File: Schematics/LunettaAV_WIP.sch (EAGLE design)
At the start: 26 parts, among them IC1 4046N, IC2 4094N, IC3 TLC339P, IC4 7805T, U1 LM358

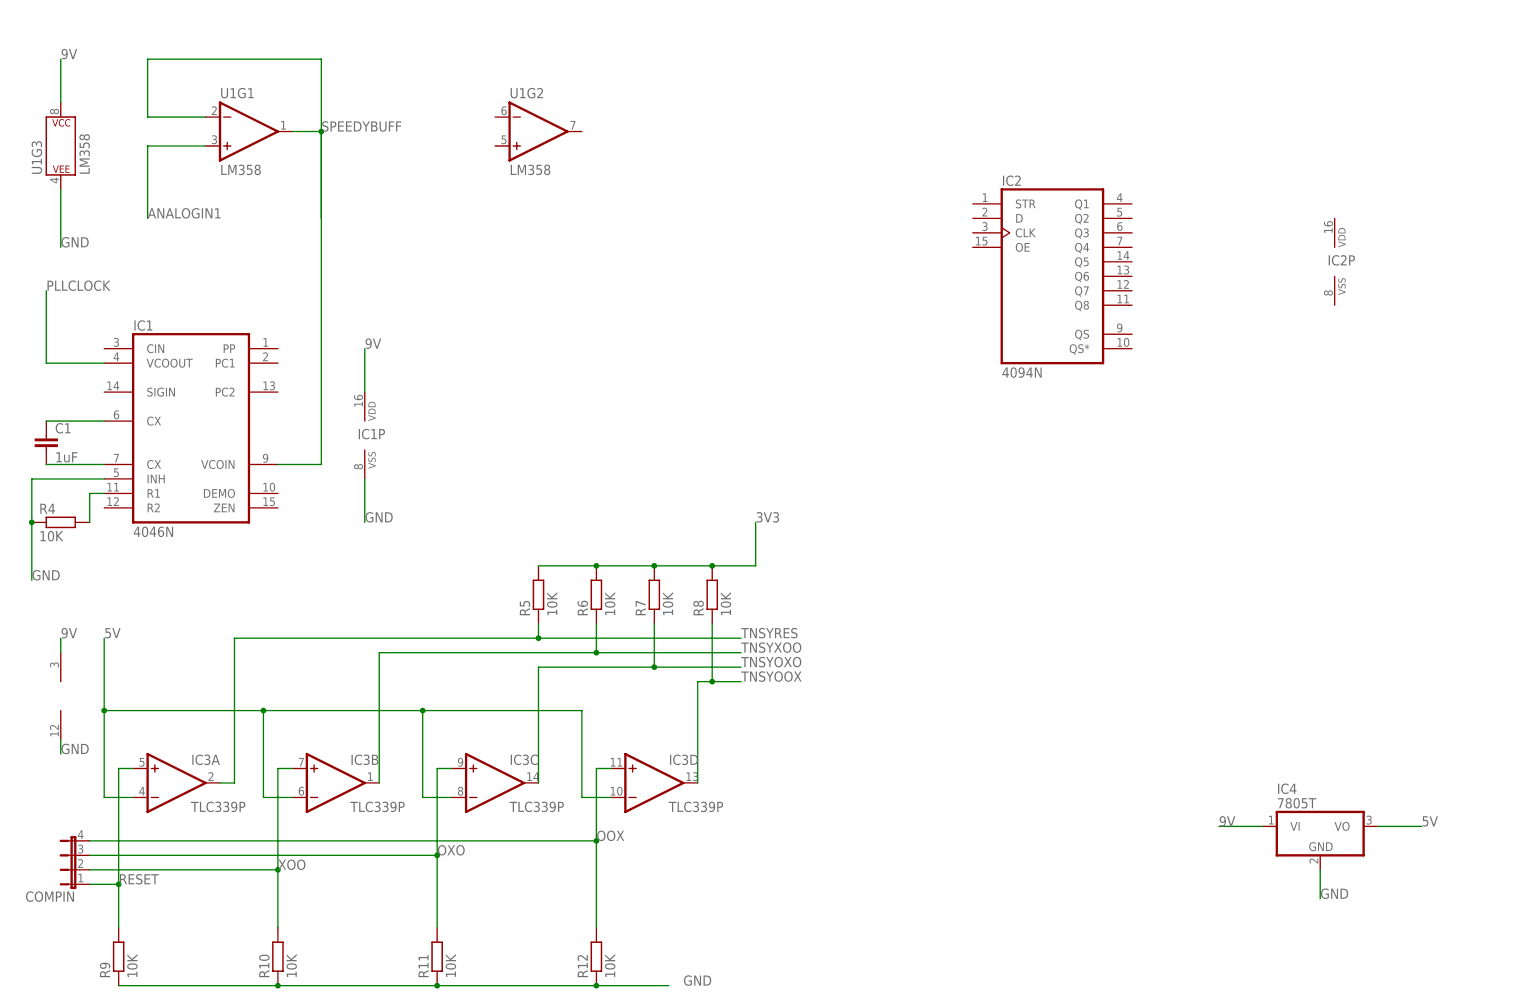
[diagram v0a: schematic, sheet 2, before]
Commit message: Add 4094, 4017, 4040 and 4051 sections
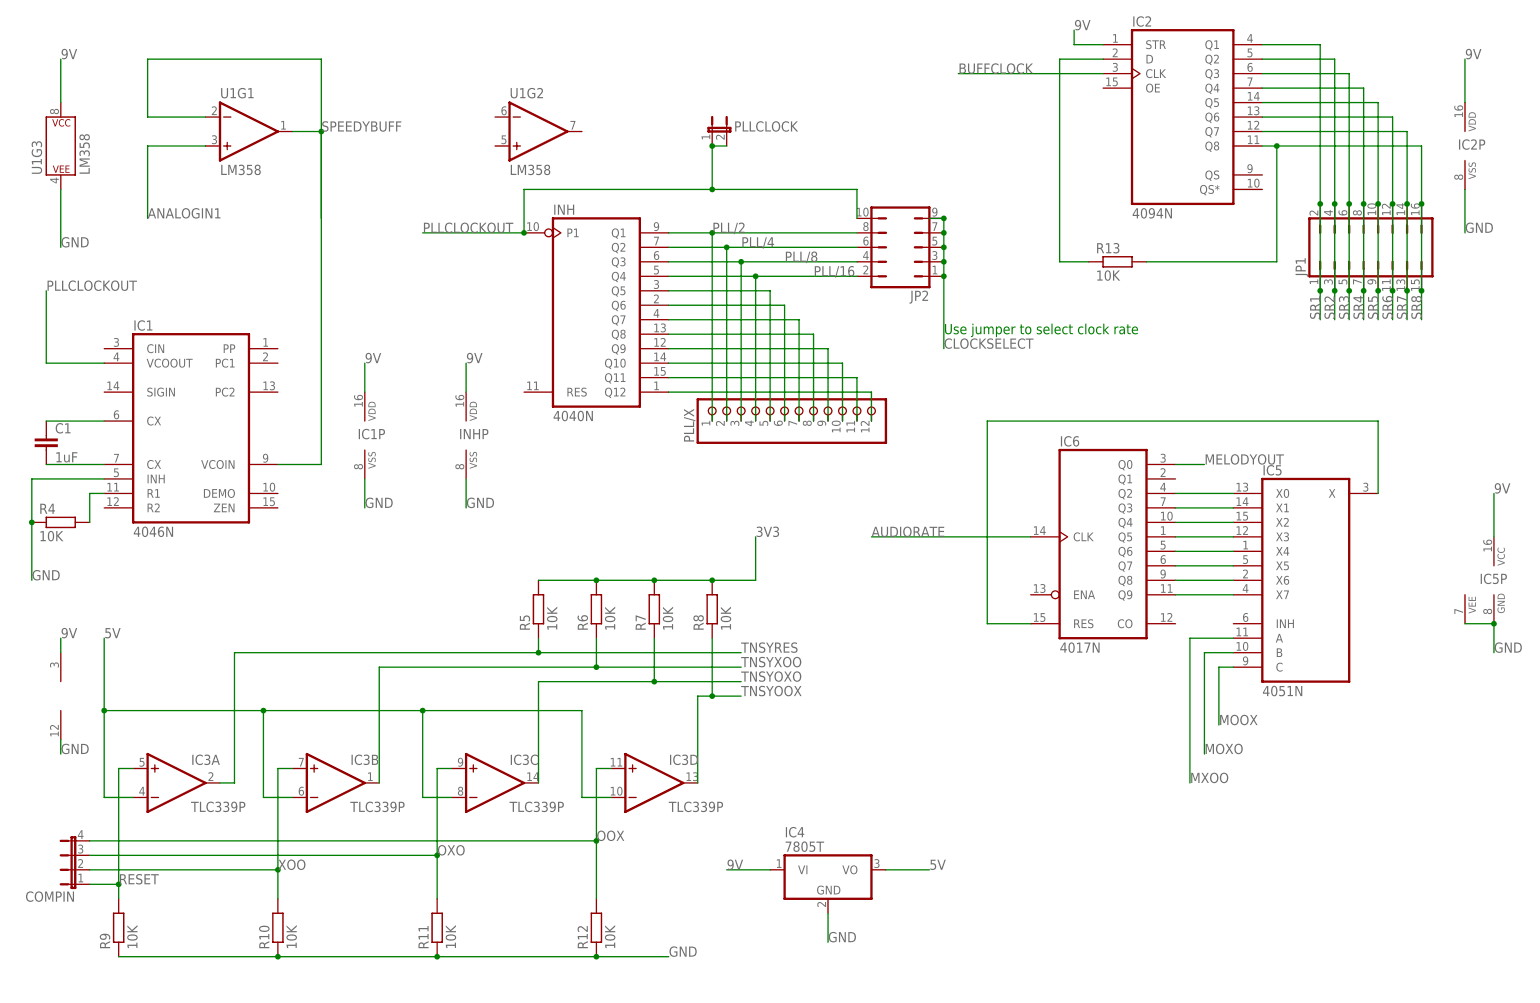
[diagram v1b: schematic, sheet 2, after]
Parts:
- added IC5: 4051N, 40xx:4051N
- added IC6: 4017N, 40xx:4017N
- added INH: 4040N, 40xx:4040N
- added JP1: (no value), jumper:JP8Q
- added JP2: (no value), jumper:JP5Q
- added PLL/X: (no value), adafruit:PINHD-1X12
- added PLLCLOCK: (no value), jumper:JP1E
- added R13: 10K, MusicThingModular:RESISTOR7MM
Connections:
- removed net PLLCLOCK: IC1A.VCOOUT
- new net AUDIORATE: IC6A.CLK
- new net BUFFCLOCK: IC2A.CLK
- new net CLOCKSELECT: JP2.1, JP2.3, JP2.5, JP2.7, JP2.9
- new net MELODYOUT: IC6A.Q0
- new net MOOX: IC5A.C
- new net MOXO: IC5A.B
- new net MXOO: IC5A.A
- new net N$11: INHA.Q5, PLL/X.5
- new net N$12: INHA.Q6, PLL/X.6
- new net N$13: INHA.Q7, PLL/X.7
- new net N$14: INHA.Q8, PLL/X.8
- new net N$15: INHA.Q9, PLL/X.9
- new net N$16: INHA.Q10, PLL/X.10
- new net N$17: INHA.Q11, PLL/X.11
- new net N$18: INHA.Q12, PLL/X.12
- new net N$19: IC5A.X, IC6A.RES
- new net N$20: IC5A.X0, IC6A.Q2
- new net N$21: IC5A.X1, IC6A.Q3
- new net N$22: IC5A.X2, IC6A.Q4
- new net N$23: IC5A.X3, IC6A.Q5
- new net N$24: IC5A.X4, IC6A.Q6
- new net N$25: IC5A.X5, IC6A.Q7
- new net N$26: IC5A.X6, IC6A.Q8
- new net N$27: IC5A.X7, IC6A.Q9
- new net N$28: IC2A.D, R13.1
- new net PLL/16: INHA.Q4, JP2.2, PLL/X.4
- new net PLL/2: INHA.Q1, JP2.8, PLL/X.1
- new net PLL/4: INHA.Q2, JP2.6, PLL/X.2
- new net PLL/8: INHA.Q3, JP2.4, PLL/X.3
- new net PLLCLOCKOUT: IC1A.VCOOUT, INHA.P1, JP2.10, PLLCLOCK.1, PLLCLOCK.2
- new net SR1: IC2A.Q1, JP1.1, JP1.2
- new net SR2: IC2A.Q2, JP1.3, JP1.4
- new net SR3: IC2A.Q3, JP1.5, JP1.6
- new net SR4: IC2A.Q4, JP1.7, JP1.8
- new net SR5: IC2A.Q5, JP1.10, JP1.9
- new net SR6: IC2A.Q6, JP1.11, JP1.12
- new net SR7: IC2A.Q7, JP1.13, JP1.14
- new net SR8: IC2A.Q8, JP1.15, JP1.16, R13.2
- net 9V: now also IC2A.STR, IC2P.VDD, IC5P.VCC, INHP.VDD
- net GND: now also IC2P.VSS, IC5P.GND, IC5P.VEE, INHP.VSS
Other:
- note added: "Use jumper to select clock rate"
- moved on the sheet: IC2, IC2P, IC4, R10, R11, R12, R5, R6, R7, R8, R9

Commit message: fix 4051 issues
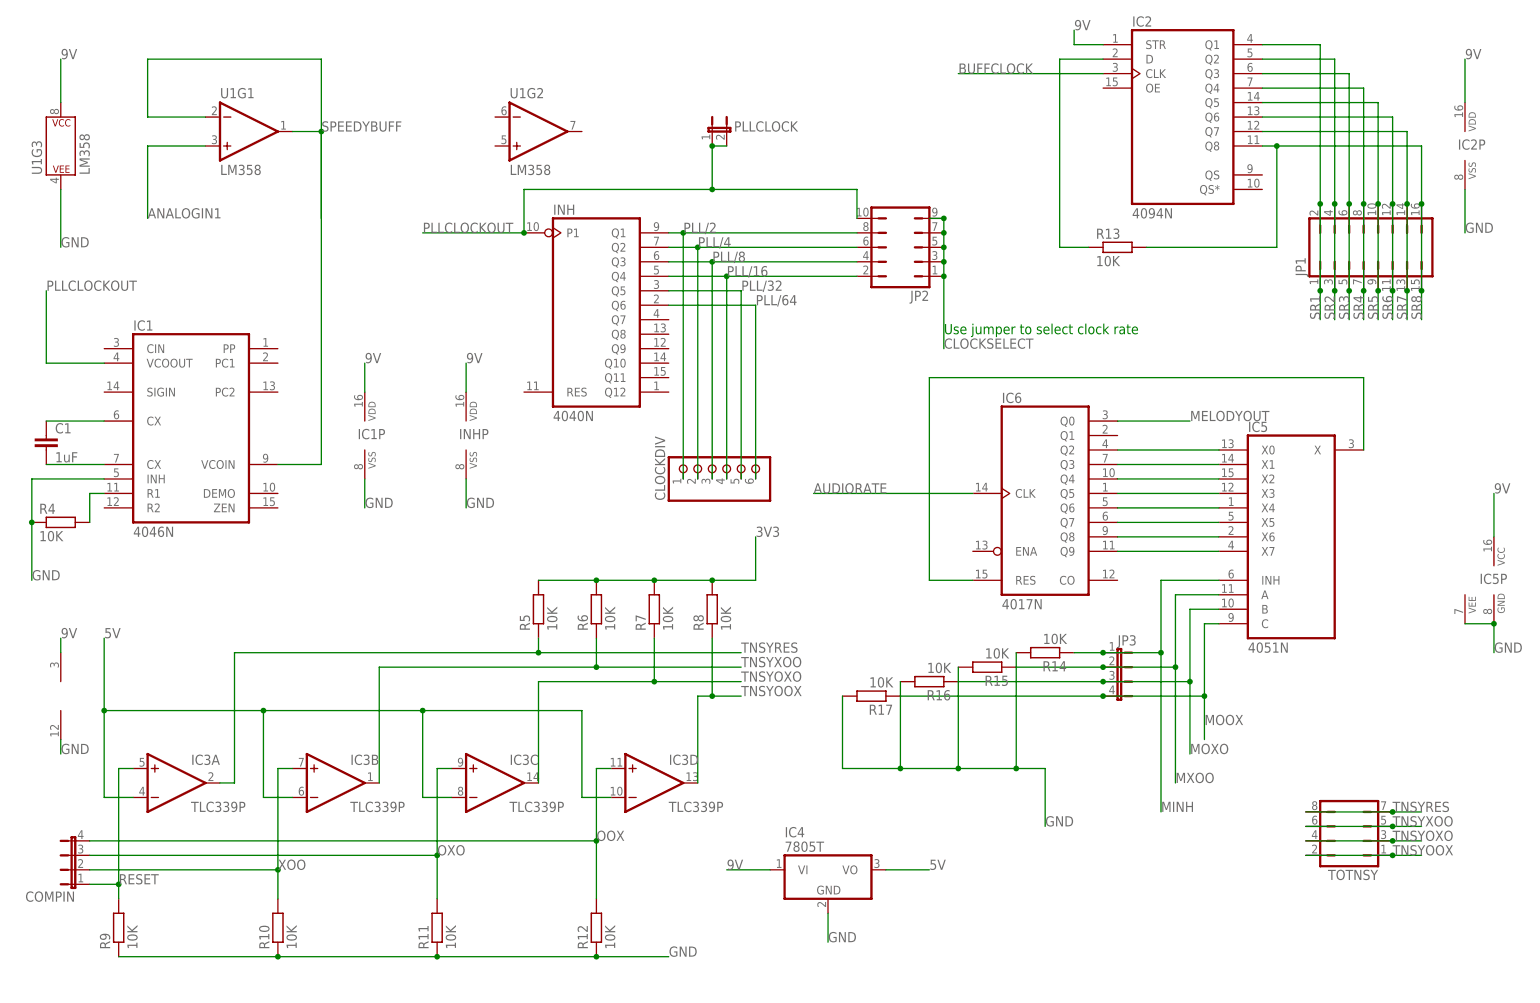
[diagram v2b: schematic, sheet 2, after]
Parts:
- removed PLL/X: (no value), adafruit:PINHD-1X12
- added CLOCKDIV: (no value), adafruit:PINHD-1X6
- added JP3: (no value), jumper:JP4E
- added R14, R15, R16, R17: 10K, MusicThingModular:RESISTOR7MM
- added TOTNSY: (no value), jumper:JP4Q
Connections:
- removed net N$11: INHA.Q5, PLL/X.5
- removed net N$12: INHA.Q6, PLL/X.6
- removed net N$13: INHA.Q7, PLL/X.7
- removed net N$14: INHA.Q8, PLL/X.8
- removed net N$15: INHA.Q9, PLL/X.9
- removed net N$16: INHA.Q10, PLL/X.10
- removed net N$17: INHA.Q11, PLL/X.11
- removed net N$18: INHA.Q12, PLL/X.12
- new net MINH: IC5A.INH, JP3.1, R14.1
- new net PLL/32: CLOCKDIV.5, INHA.Q5
- new net PLL/64: CLOCKDIV.6, INHA.Q6
- net GND: now also R14.2, R15.2, R16.2, R17.2
- net MOOX: now also JP3.4, R17.1
- net MOXO: now also JP3.3, R16.1
- net MXOO: now also JP3.2, R15.1
- net PLL/16: now also CLOCKDIV.4; no longer PLL/X.4
- net PLL/2: now also CLOCKDIV.1; no longer PLL/X.1
- net PLL/4: now also CLOCKDIV.2; no longer PLL/X.2
- net PLL/8: now also CLOCKDIV.3; no longer PLL/X.3
- net TNSYOOX: now also TOTNSY.1, TOTNSY.2
- net TNSYOXO: now also TOTNSY.3, TOTNSY.4
- net TNSYRES: now also TOTNSY.7, TOTNSY.8
- net TNSYXOO: now also TOTNSY.5, TOTNSY.6
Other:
- moved on the sheet: IC5, IC6, R13
